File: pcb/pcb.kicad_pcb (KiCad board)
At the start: 2 copper layers, 234.6 x 93.6 mm, 85 parts, among them SW1 SW_PUSH, SW10 SW_PUSH, SW11 SW_PUSH, SW12 SW_PUSH, SW13 SW_PUSH, SW14 SW_PUSH, SW15 SW_PUSH, SW16 SW_PUSH, SW17 SW_PUSH, SW18 SW_PUSH, SW19 SW_PUSH, SW2 SW_PUSH, SW20 SW_PUSH, SW21 SW_PUSH, SW22 SW_PUSH, SW23 SW_PUSH, SW24 SW_PUSH, SW25 SW_PUSH, SW26 SW_PUSH, SW27 SW_PUSH, SW28 SW_PUSH, SW29 SW_PUSH, SW3 SW_PUSH, SW30 SW_PUSH, SW31 SW_PUSH, SW32 SW_PUSH, SW33 SW_DPST, SW34 SW_PUSH, SW4 SW_PUSH, SW5 SW_PUSH, SW6 SW_PUSH, SW7 SW_PUSH, SW8 SW_PUSH, SW9 SW_PUSH, U1 ProMicro

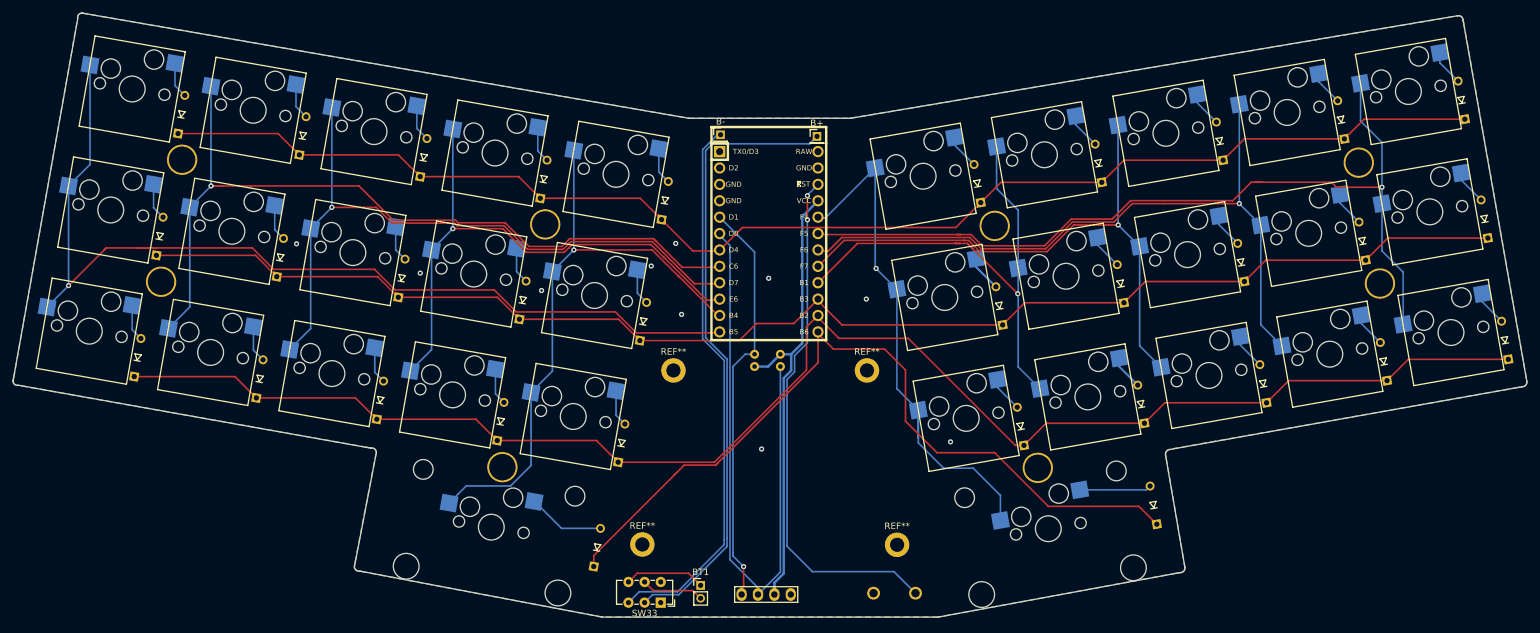
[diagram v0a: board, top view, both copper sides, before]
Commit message: Add files via upload
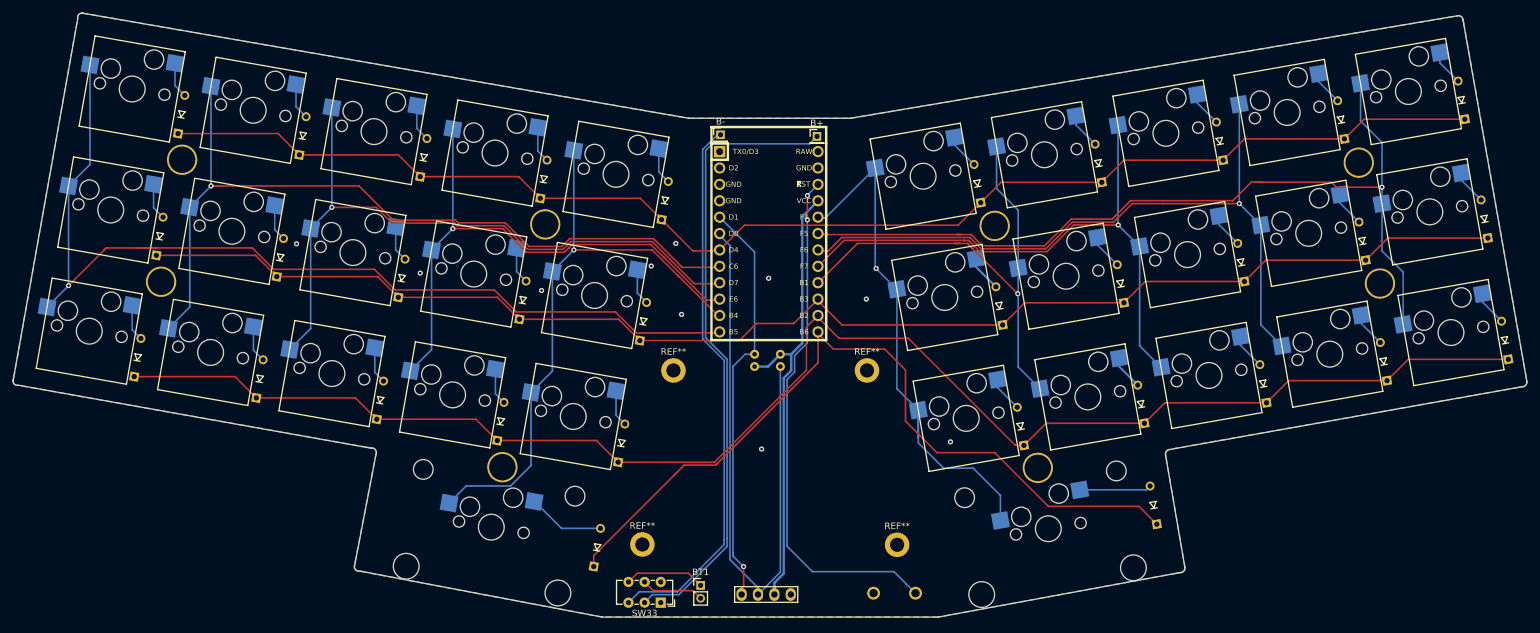
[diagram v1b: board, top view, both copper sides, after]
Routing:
- net (no net): track 183.5 -> 1.16 mm
- net +BATT: track 0.00 -> 97.4 mm
- net -BATT: track 0.00 -> 84.9 mm
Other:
- net class Default removed
- net class Power removed
